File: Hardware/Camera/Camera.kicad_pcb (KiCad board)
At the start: 4 copper layers, 46.7 x 75.9 mm, 65 parts, among them J1 Power, J2 ICC Out, J3 USB_B_Mini, J4 SWDIO, J5 Header Pins, J6 Camer Interface, Q1 AO3401A, SW1 SW_SPDT, U1 STM32F407ZGT6, U2 LM317L_SOT-89, U3 LM317L_SOT-89, Y1 16MHz

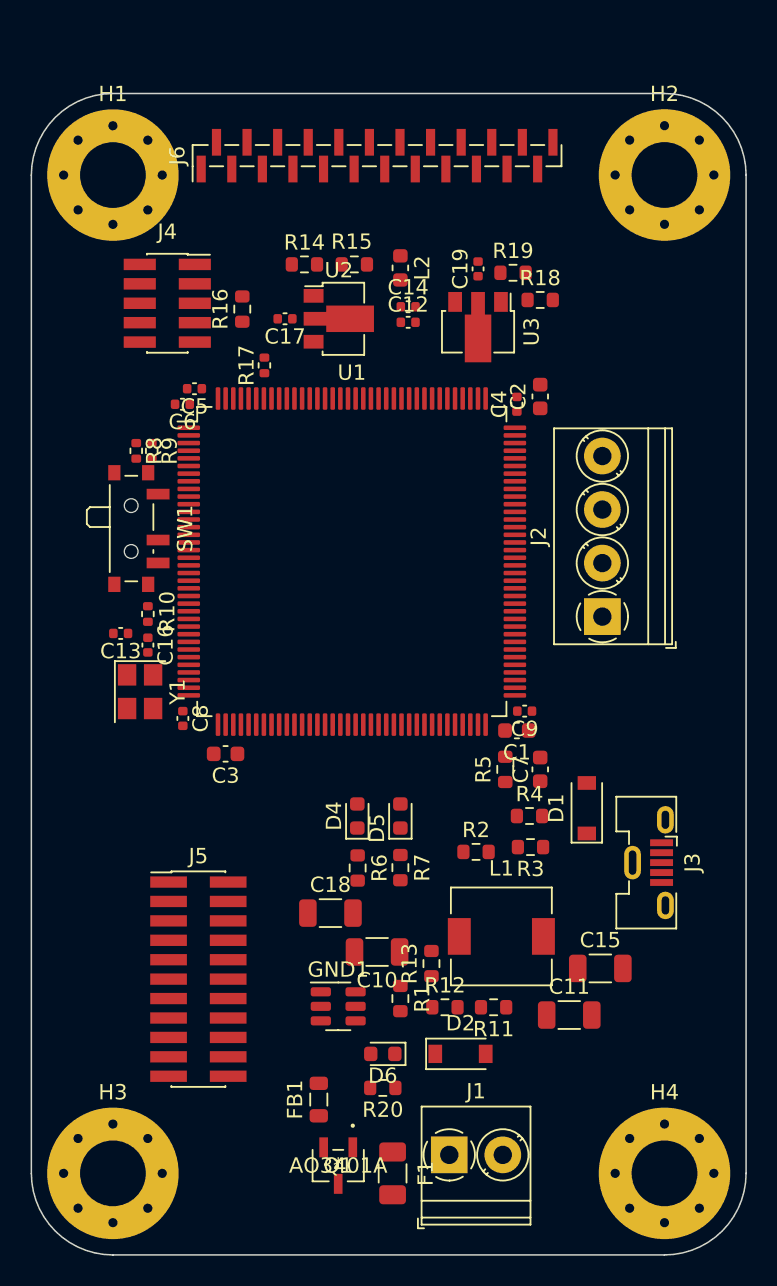
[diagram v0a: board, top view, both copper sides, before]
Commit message: Finished initial placement
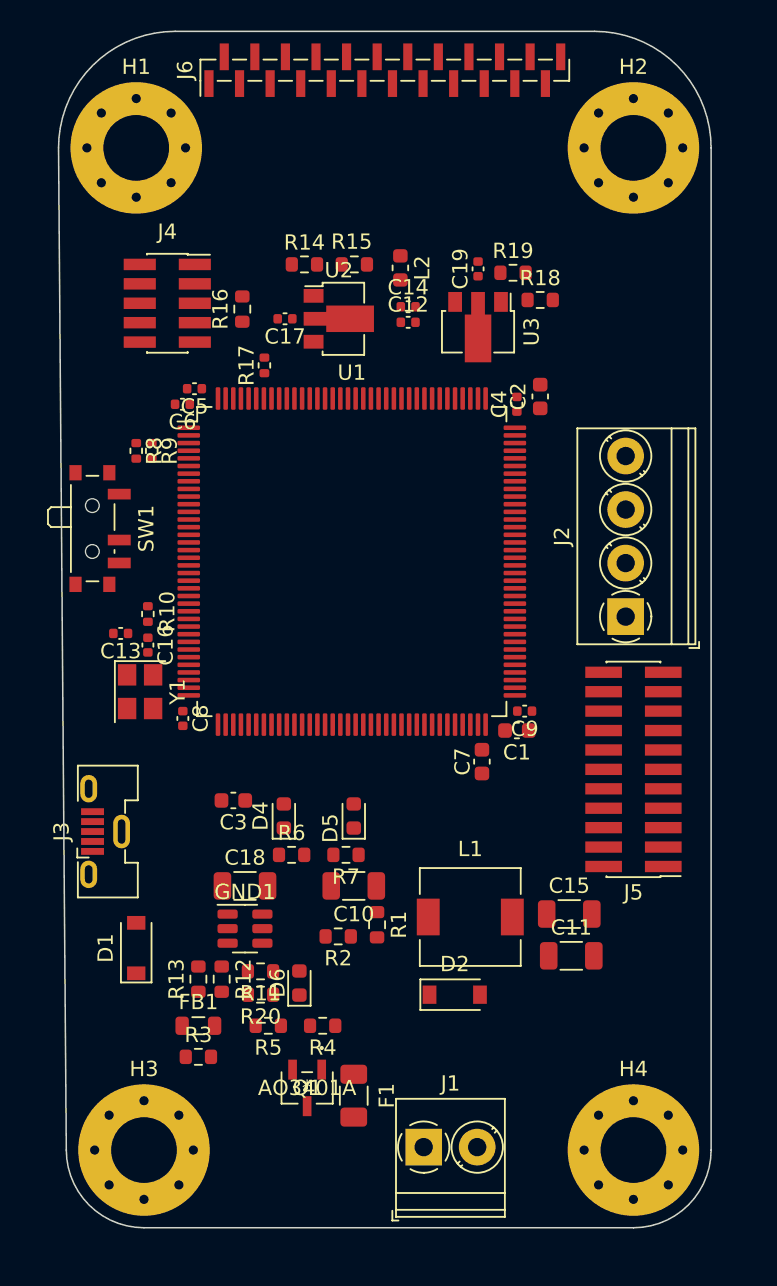
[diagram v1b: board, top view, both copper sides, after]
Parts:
- moved J3 35.6 mm to (120.4, 107.2), turned to 90 degrees
- moved J5 31.6 mm to (154.9, 103.1), turned to 180 degrees
- moved D1 30.9 mm to (122.4, 114.8)
- moved R3 25.7 mm to (126.5, 121.9), turned to 0 degrees
- moved R5 22.8 mm to (131.1, 119.9), turned to 180 degrees
- moved R4 19.3 mm to (134.6, 119.9), turned to 180 degrees
- moved R11 15.4 mm to (130.6, 116.3)
- moved R13 15.3 mm to (126.5, 116.8)
- moved R12 14.7 mm to (128.0, 116.8), turned to -90 degrees
- moved R2 10.6 mm to (135.6, 114.0), turned to 180 degrees
- moved R20 10.1 mm to (130.6, 117.9)
- moved FB1 9.24 mm to (126.5, 119.9), turned to 0 degrees
- moved GND1 7.94 mm to (129.5, 113.5)
- moved D6 7.16 mm to (133.1, 117.1), turned to 90 degrees
- moved C18 5.86 mm to (129.5, 110.7)
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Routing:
- removed copper zone on In2.Cu, net +3.3VA
- removed copper zone on In1.Cu, net GND
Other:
- board size 46.7 x 75.9 mm -> 42.7 x 78.2 mm
